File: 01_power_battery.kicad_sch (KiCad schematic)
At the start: 210 parts, among them Q13 CSD19537Q3 100V AUX reverse F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, Q14 BSS138 fast reverse-gate pull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, Q21 SiSS4409DN 40V reverse-blocki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, Q22 SiSS4409DN 40V reverse-blocki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, Q23 SiSS4409DN 40V reverse-blocki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, Q24 SiSS4409DN 40V reverse-blocki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, Q25 CSD17575Q3 battery power-path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, Q26 SiSS4409DN 40V reverse-blocki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, Q2600 CSD17577Q3A 30V switching FET, Q2601 CSD17577Q3A 30V switching FET, Q2602 CSD17577Q3A 30V switching FET, Q2603 CSD17577Q3A 30V switching FET, Q2604 BSS138, Q2605 BSS138, Q2620 CSD19537Q3 100V, Q2621 CSD19537Q3 100V, Q2622 CSD19537Q3 100V, Q2623 CSD19537Q3 100V, Q2644 BSS138 AUX discharge, Q2650 CSD19537Q3 100V, Q2660 CSD18540Q5B AON pass FET, Q27 SiSS4409DN 40V reverse-blocki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, Q28 SiSS4409DN 40V reverse-blocki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, Q29 SiSS4409DN 40V reverse-blocki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, Q700 BSS138, Q702 BSS138, U10 BQ34Z100-G1 protected-pack ga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, U12 TPS26630RGER 3A AUX eFuse / s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, U15 LTC4418IUF#PBF dual-input sel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, U16 LTC4418IUF#PBF dual-input sel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, U2 ISL9241IRTZ, U2620 LM74700QDBVRQ1, U2621 LM74700QDBVRQ1, U2634 TPS3700DDCR charger-bias dete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, U2635 TCA9537DGSR power status and 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, U2644 SN74LVC1G04DBVR AUX discharge, U2650 LM74700QDBVRQ1 system standby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, U2660 LTC4231IMS-1#PBF standby curr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, U718 LTC4368IMS-2#PBF standby brea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

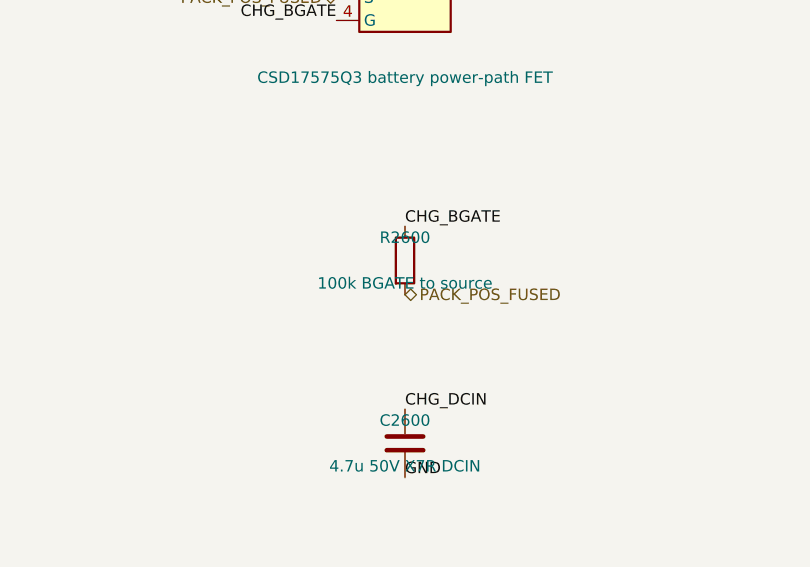
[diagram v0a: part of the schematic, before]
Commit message: finish the keyboard and update the case and power
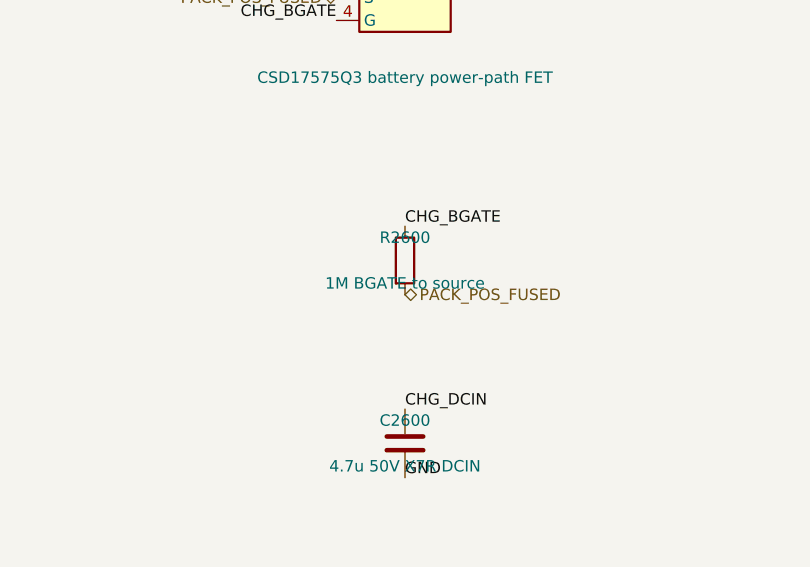
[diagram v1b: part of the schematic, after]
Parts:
- C2606: MPN GRM188R71H473KA61D -> C0603C473K5RACTU; Manufacturer Murata -> KEMET
- C720: MPN GRM21BR71H105KA01 -> C2012X7R1H105K125AB; Manufacturer Murata -> TDK
- R2600: value 100k BGATE to source -> 1M BGATE to source; MPN RC0603FR-07100KL -> RC0603FR-071ML
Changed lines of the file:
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@@
   (dnp no)
   (property "Reference" "R2600" (at 1089.66 237.49 0) (effects (font (size 1.27 1.27))))
-  (property "Value" "100k BGATE to source" (at 1089.66 242.57 0) (effects (font (size 1.27 1.27))))
+  (property "Value" "1M BGATE to source" (at 1089.66 242.57 0) (effects (font (size 1.27 1.27))))
   (property "Footprint" "Resistor_SMD:R_0603_1608Metric" (at 1089.66 240.03 0) (effects (font (size 1.27 1.27)) (hide yes)))
   (property "Datasheet" "" (at 1089.66 240.03 0) (effects (font (size 1.27 1.27)) (hide yes)))
   (property "Manufacturer" "Yageo" (at 1089.66 240.03 0) (effects (font (size 1.27 1.27)) (hide yes)))
-  (property "MPN" "RC0603FR-07100KL" (at 1089.66 240.03 0) (effects (font (size 1.27 1.27)) (hide yes)))
+  (property "MPN" "RC0603FR-071ML" (at 1089.66 240.03 0) (effects (font (size 1.27 1.27)) (hide yes)))
   (pin "1")
   (pin "2")
@@
   (property "Footprint" "Capacitor_SMD:C_0603_1608Metric" (at 1089.66 384.81 0) (effects (font (size 1.27 1.27)) (hide yes)))
   (property "Datasheet" "" (at 1089.66 384.81 0) (effects (font (size 1.27 1.27)) (hide yes)))
-  (property "Manufacturer" "Murata" (at 1089.66 384.81 0) (effects (font (size 1.27 1.27)) (hide yes)))
-  (property "MPN" "GRM188R71H473KA61D" (at 1089.66 384.81 0) (effects (font (size 1.27 1.27)) (hide yes)))
+  (property "Manufacturer" "KEMET" (at 1089.66 384.81 0) (effects (font (size 1.27 1.27)) (hide yes)))
+  (property "MPN" "C0603C473K5RACTU" (at 1089.66 384.81 0) (effects (font (size 1.27 1.27)) (hide yes)))
   (pin "1")
   (pin "2")
@@
   (property "Footprint" "Capacitor_SMD:C_0805_2012Metric" (at 379.73 190.5 0) (effects (font (size 1.27 1.27)) (hide yes)))
   (property "Datasheet" "" (at 379.73 190.5 0) (effects (font (size 1.27 1.27)) (hide yes)))
-  (property "Manufacturer" "Murata" (at 379.73 190.5 0) (effects (font (size 1.27 1.27)) (hide yes)))
-  (property "MPN" "GRM21BR71H105KA01" (at 379.73 190.5 0) (effects (font (size 1.27 1.27)) (hide yes)))
+  (property "Manufacturer" "TDK" (at 379.73 190.5 0) (effects (font (size 1.27 1.27)) (hide yes)))
+  (property "MPN" "C2012X7R1H105K125AB" (at 379.73 190.5 0) (effects (font (size 1.27 1.27)) (hide yes)))
   (pin "1")
   (pin "2")
